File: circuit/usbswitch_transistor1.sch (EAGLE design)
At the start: 11 parts, among them IC1 TINY25, Q2 BSA223SP

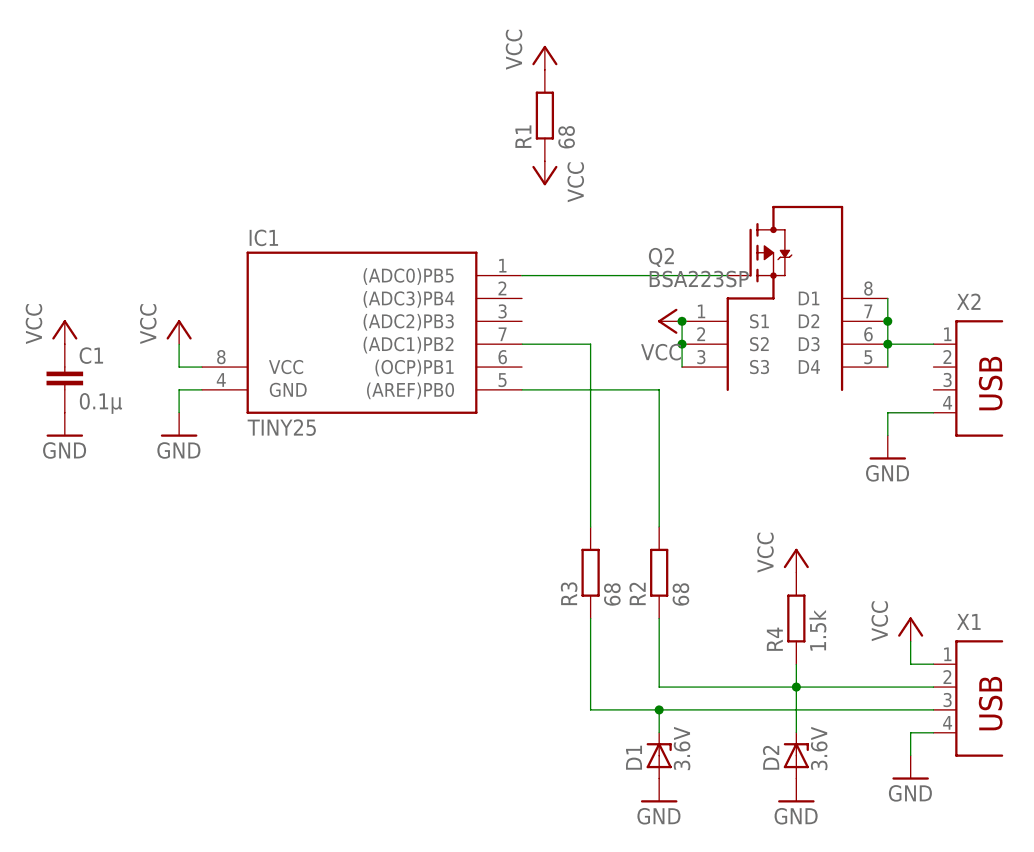
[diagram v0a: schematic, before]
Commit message: SMD-Varianten
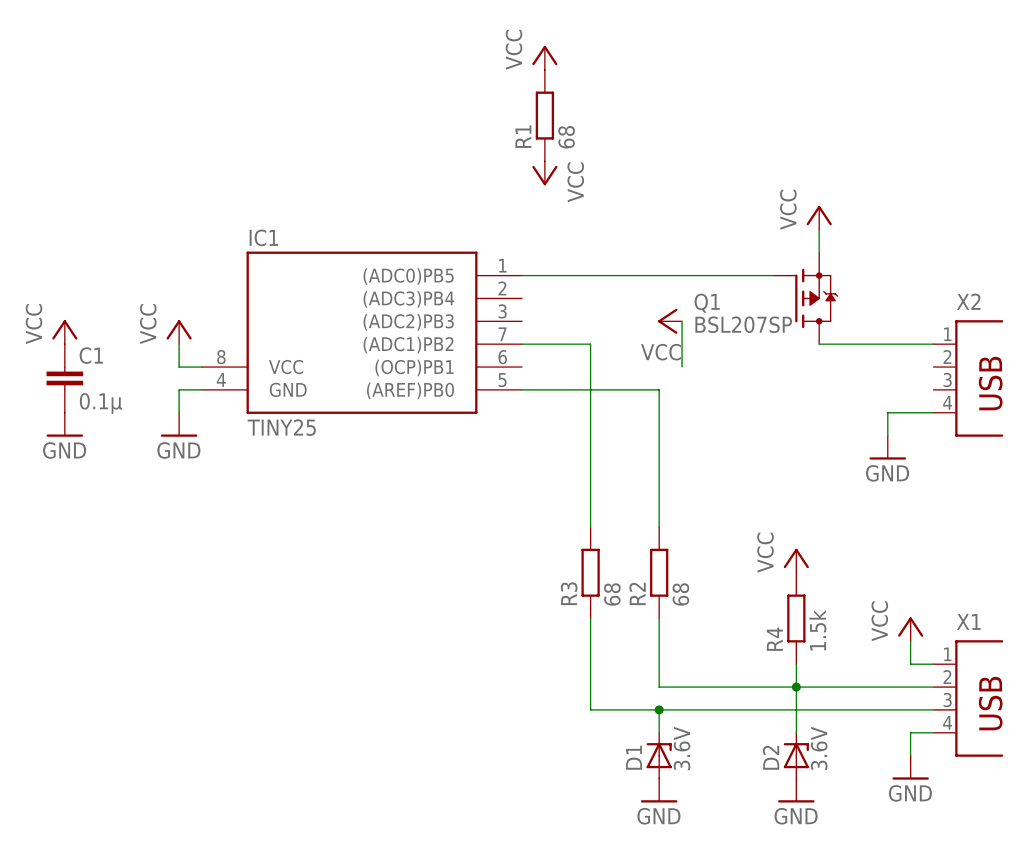
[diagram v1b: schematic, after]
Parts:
- removed Q2: BSA223SP, irf:BSA223SP
- added Q1: BSL207SP, irf:BSL207SP
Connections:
- net N$1: now also Q1.G; no longer Q2.G
- net N$2: now also Q1.D; no longer Q2.D1, Q2.D2, Q2.D3, Q2.D4
- net VCC: now also Q1.S; no longer Q2.S1, Q2.S2, Q2.S3
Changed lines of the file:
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@@
 <grid distance="0.1" unitdist="inch" unit="inch" style="lines" multiple="1" display="no" altdistance="0.01" altunitdist="inch" altunit="inch"/>
 <layers>
-<layer number="1" name="Top" color="4" fill="1" visible="yes" active="no"/>
-<layer number="16" name="Bottom" color="1" fill="1" visible="yes" active="no"/>
-<layer number="17" name="Pads" color="2" fill="1" visible="yes" active="no"/>
-<layer number="18" name="Vias" color="2" fill="1" visible="yes" active="no"/>
-<layer number="19" name="Unrouted" color="6" fill="1" visible="yes" active="no"/>
-<layer number="20" name="Dimension" color="15" fill="1" visible="yes" active="no"/>
-<layer number="21" name="tPlace" color="7" fill="1" visible="yes" active="no"/>
-<layer number="22" name="bPlace" color="7" fill="1" visible="yes" active="no"/>
-<layer number="23" name="tOrigins" color="15" fill="1" visible="yes" active="no"/>
-<layer number="24" name="bOrigins" color="15" fill="1" visible="yes" active="no"/>
-<layer number="25" name="tNames" color="7" fill="1" visible="yes" active="no"/>
-<layer number="26" name="bNames" color="7" fill="1" visible="yes" active="no"/>
-<layer number="27" name="tValues" color="7" fill="1" visible="yes" active="no"/>
-<layer number="28" name="bValues" color="7" fill="1" visible="yes" active="no"/>
+<layer number="1" name="Top" color="4" fill="1" visible="no" active="no"/>
+<layer number="16" name="Bottom" color="1" fill="1" visible="no" active="no"/>
+<layer number="17" name="Pads" color="2" fill="1" visible="no" active="no"/>
+<layer number="18" name="Vias" color="2" fill="1" visible="no" active="no"/>
+<layer number="19" name="Unrouted" color="6" fill="1" visible="no" active="no"/>
+<layer number="20" name="Dimension" color="15" fill="1" visible="no" active="no"/>
+<layer number="21" name="tPlace" color="7" fill="1" visible="no" active="no"/>
+<layer number="22" name="bPlace" color="7" fill="1" visible="no" active="no"/>
+<layer number="23" name="tOrigins" color="15" fill="1" visible="no" active="no"/>
+<layer number="24" name="bOrigins" color="15" fill="1" visible="no" active="no"/>
+<layer number="25" name="tNames" color="7" fill="1" visible="no" active="no"/>
+<layer number="26" name="bNames" color="7" fill="1" visible="no" active="no"/>
+<layer number="27" name="tValues" color="7" fill="1" visible="no" active="no"/>
+<layer number="28" name="bValues" color="7" fill="1" visible="no" active="no"/>
 <layer number="29" name="tStop" color="7" fill="3" visible="no" active="no"/>
 <layer number="30" name="bStop" color="7" fill="6" visible="no" active="no"/>
@@
 <layer number="35" name="tGlue" color="7" fill="4" visible="no" active="no"/>
 <layer number="36" name="bGlue" color="7" fill="5" visible="no" active="no"/>
-<layer number="37" name="tTest" color="7" fill="1" visible="yes" active="no"/>
-<layer number="38" name="bTest" color="7" fill="1" visible="yes" active="no"/>
+<layer number="37" name="tTest" color="7" fill="1" visible="no" active="no"/>
+<layer number="38" name="bTest" color="7" fill="1" visible="no" active="no"/>
 <layer number="39" name="tKeepout" color="4" fill="11" visible="no" active="no"/>
 <layer number="40" name="bKeepout" color="1" fill="11" visible="no" active="no"/>
@@
 <layer number="44" name="Drills" color="7" fill="1" visible="no" active="no"/>
 <layer number="45" name="Holes" color="7" fill="1" visible="no" active="no"/>
-<layer number="46" name="Milling" color="3" fill="1" visible="yes" active="no"/>
-<layer number="47" name="Measures" color="7" fill="1" visible="yes" active="no"/>
-<layer number="48" name="Document" color="7" fill="1" visible="yes" active="no"/>
-<layer number="49" name="Reference" color="7" fill="1" visible="yes" active="no"/>
-<layer number="51" name="tDocu" color="7" fill="1" visible="yes" active="no"/>
-<layer number="52" name="bDocu" color="7" fill="1" visible="yes" active="no"/>
+<layer number="46" name="Milling" color="3" fill="1" visible="no" active="no"/>
+<layer number="47" name="Measures" color="7" fill="1" visible="no" active="no"/>
+<layer number="48" name="Document" color="7" fill="1" visible="no" active="no"/>
+<layer number="49" name="Reference" color="7" fill="1" visible="no" active="no"/>
+<layer number="51" name="tDocu" color="7" fill="1" visible="no" active="no"/>
+<layer number="52" name="bDocu" color="7" fill="1" visible="no" active="no"/>
 <layer number="91" name="Nets" color="2" fill="1" visible="yes" active="yes"/>
 <layer number="92" name="Busses" color="1" fill="1" visible="yes" active="yes"/>
@@
 <part name="GND7" library="supply1" deviceset="GND" device=""/>
 <part name="C1" library="resistor" deviceset="C-EU" device="C1206" value="0.1µ"/>
-<part name="Q2" library="irf" deviceset="BSA223SP" device=""/>
 <part name="R1" library="resistor" deviceset="R-EU_" device="R1206" value="68"/>
 <part name="P+5" library="supply1" deviceset="VCC" device=""/>
 <part name="P+7" library="supply1" deviceset="VCC" device=""/>
+<part name="Q1" library="irf" deviceset="BSL207SP" device=""/>
+<part name="P+8" library="supply1" deviceset="VCC" device=""/>
 </parts>
 <sheets>
@@
 <instance part="GND7" gate="1" x="25.4" y="58.42"/>
 <instance part="C1" gate="G$1" x="25.4" y="66.04"/>
-<instance part="Q2" gate="G$1" x="101.6" y="78.74"/>
 <instance part="R1" gate="G$1" x="78.74" y="93.98" rot="R90"/>
 <instance part="P+5" gate="VCC" x="78.74" y="101.6"/>
 <instance part="P+7" gate="VCC" x="78.74" y="86.36" rot="R180"/>
+<instance part="Q1" gate="G$1" x="106.68" y="73.66"/>
+<instance part="P+8" gate="VCC" x="109.22" y="83.82"/>
 </instances>
 <busses>
@@
 </segment>
 <segment>
-<pinref part="Q2" gate="G$1" pin="S1"/>
 <pinref part="P+3" gate="VCC" pin="VCC"/>
-<pinref part="Q2" gate="G$1" pin="S3"/>
-<wire x1="93.98" y1="71.12" x2="93.98" y2="68.58" width="0.1524" layer="91"/>
-<junction x="93.98" y="71.12"/>
-<pinref part="Q2" gate="G$1" pin="S2"/>
-<wire x1="93.98" y1="68.58" x2="93.98" y2="66.04" width="0.1524" layer="91"/>
-<junction x="93.98" y="68.58"/>
+<wire x1="93.98" y1="71.12" x2="93.98" y2="66.04" width="0.1524" layer="91"/>
 </segment>
 <segment>
@@
 <pinref part="P+7" gate="VCC" pin="VCC"/>
 </segment>
+<segment>
+<pinref part="Q1" gate="G$1" pin="S"/>
+<pinref part="P+8" gate="VCC" pin="VCC"/>
+<wire x1="109.22" y1="81.28" x2="109.22" y2="78.74" width="0.1524" layer="91"/>
+</segment>
 </net>
 <net name="N$1" class="0">
 <segment>
 <pinref part="IC1" gate="G$1" pin="(ADC0)PB5"/>
-<wire x1="99.06" y1="76.2" x2="76.2" y2="76.2" width="0.1524" layer="91"/>
-<pinref part="Q2" gate="G$1" pin="G"/>
+<wire x1="104.14" y1="76.2" x2="76.2" y2="76.2" width="0.1524" layer="91"/>
+<pinref part="Q1" gate="G$1" pin="G"/>
 </segment>
 </net>
@@
 <net name="N$2" class="0">
 <segment>
-<pinref part="Q2" gate="G$1" pin="D1"/>
-<pinref part="Q2" gate="G$1" pin="D4"/>
-<wire x1="116.84" y1="73.66" x2="116.84" y2="71.12" width="0.1524" layer="91"/>
-<pinref part="Q2" gate="G$1" pin="D2"/>
-<wire x1="116.84" y1="71.12" x2="116.84" y2="68.58" width="0.1524" layer="91"/>
-<junction x="116.84" y="71.12"/>
-<pinref part="Q2" gate="G$1" pin="D3"/>
-<wire x1="116.84" y1="68.58" x2="116.84" y2="66.04" width="0.1524" layer="91"/>
-<junction x="116.84" y="68.58"/>
+<pinref part="Q1" gate="G$1" pin="D"/>
 <pinref part="X2" gate="G$1" pin="1"/>
-<wire x1="116.84" y1="68.58" x2="121.92" y2="68.58" width="0.1524" layer="91"/>
-</segment>
-</net>
+<wire x1="109.22" y1="68.58" x2="121.92" y2="68.58" width="0.1524" layer="91"/>
+</segment>
+</net>
